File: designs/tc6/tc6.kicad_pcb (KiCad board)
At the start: 2 copper layers, 59.2 x 26.5 mm, 19 parts, among them J1001 SSM-104-L-SV, P1 TC2030, U1001 MCP6001-OT

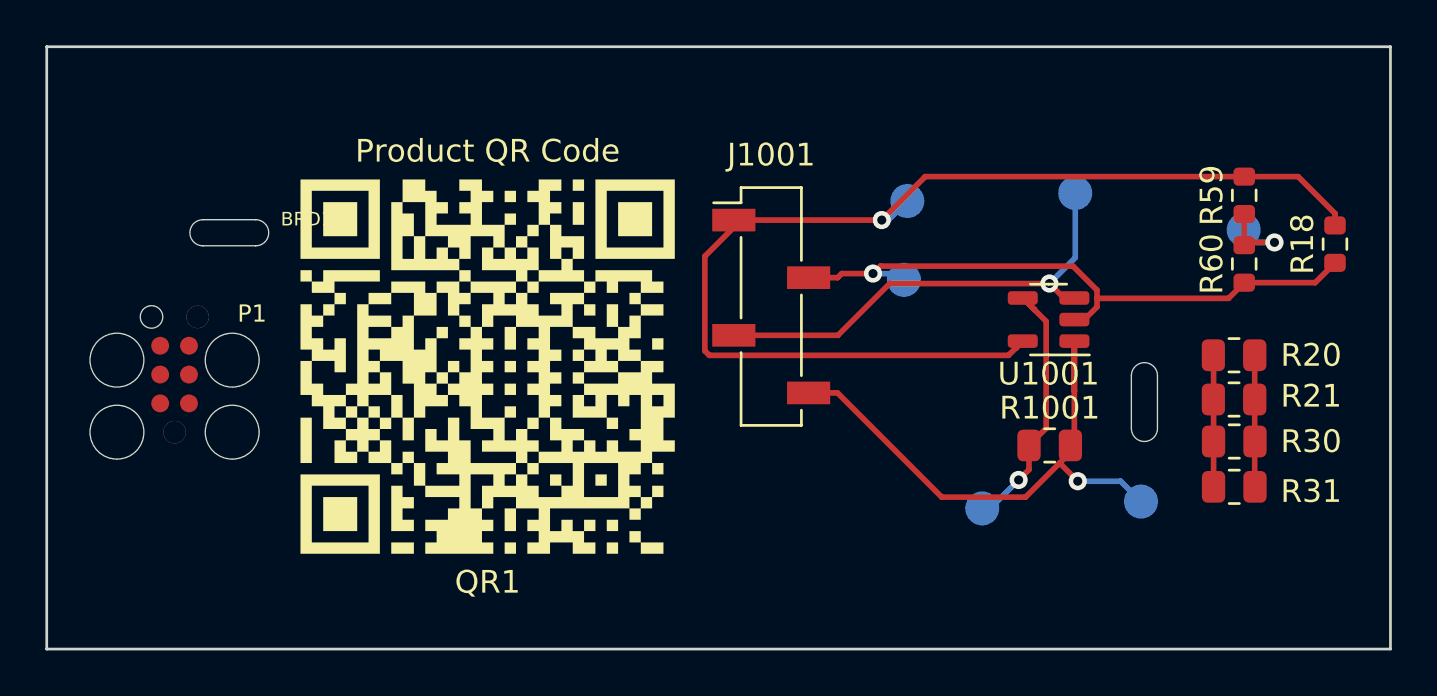
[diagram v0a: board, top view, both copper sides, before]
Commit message: Update to kicad6
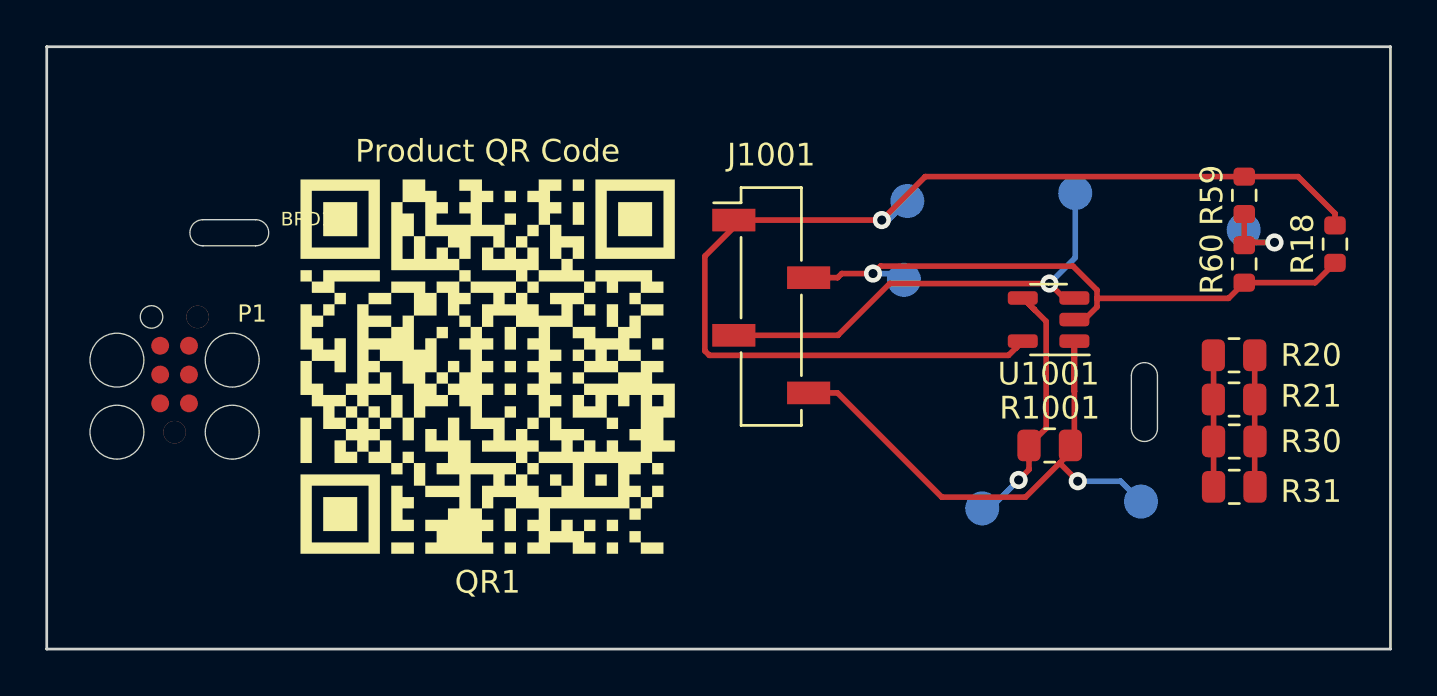
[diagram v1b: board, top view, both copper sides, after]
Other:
- net class Default removed

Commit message: migrating to version6
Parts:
- BRD1: footprint tc5:DemoBoard -> tc6:DemoBoard
- P1: footprint tc5:TC2030-MCP-FP -> tc6:TC2030-MCP-FP
- QR1: footprint tc5:TC5 -> tc6:TC5
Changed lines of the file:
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@@
     )
   )
-  (footprint "tc5:TC5" (layer "F.Cu")
+  (footprint "tc6:TC5" (layer "F.Cu")
     (at 135.3 97.9)
     (attr through_hole)
@@
     )
   )
-  (footprint "tc5:DemoBoard" (layer "F.Cu")
+  (footprint "tc6:DemoBoard" (layer "F.Cu")
     (at 127.325 91.1)
     (attr through_hole)
@@
     )
   )
-  (footprint "tc5:TC2030-MCP-FP" (layer "F.Cu")
+  (footprint "tc6:TC2030-MCP-FP" (layer "F.Cu")
     (at 121.5 98.25 90)
     (descr "http://www.tag-connect.com/Materials/TC2030-MCP%20PCB%20Footprint.pdf")

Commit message: Step 1 for Test case demonstrating difference shift based on viewed layers
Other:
- board text added: "Dummy text"
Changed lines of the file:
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@@
   (gr_line (start 164.825 100.625) (end 164.825 98.3) (layer "Edge.Cuts") (width 0.05))
   (gr_arc (start 122.75 92.575) (mid 122.175 92) (end 122.75 91.425) (layer "Edge.Cuts") (width 0.05))
+  (gr_text "Dummy text" (at 196.59 93) (layer "B.SilkS")
+    (effects (font (size 1 1) (thickness 0.15)))
+  )
   (dimension (type aligned) (layer "Dwgs.User")
     (pts (xy 175.095 110.35) (xy 115.865 110.35))
